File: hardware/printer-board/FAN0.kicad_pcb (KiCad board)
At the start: 2 copper layers, 100 x 100 mm, 12 parts, among them J33 TO FAN0, Q4 D882

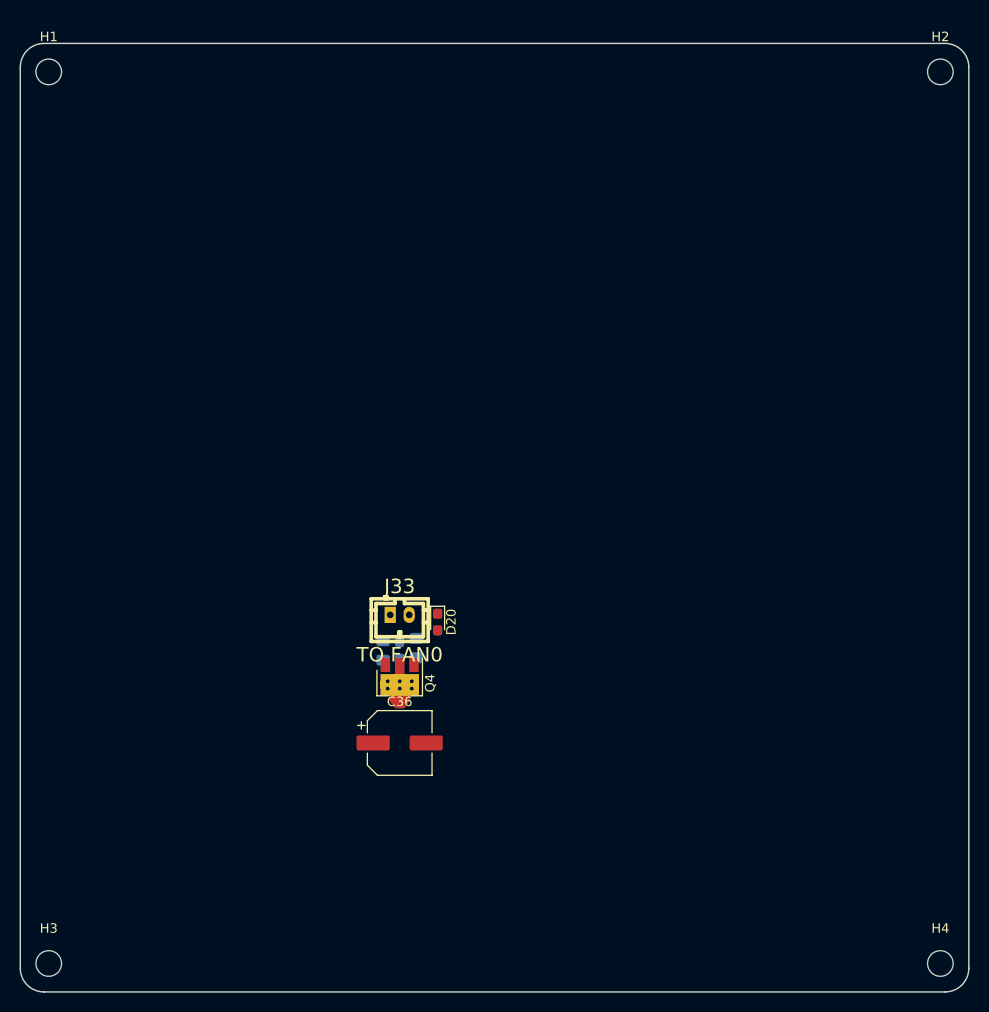
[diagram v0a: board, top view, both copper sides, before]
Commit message: update,
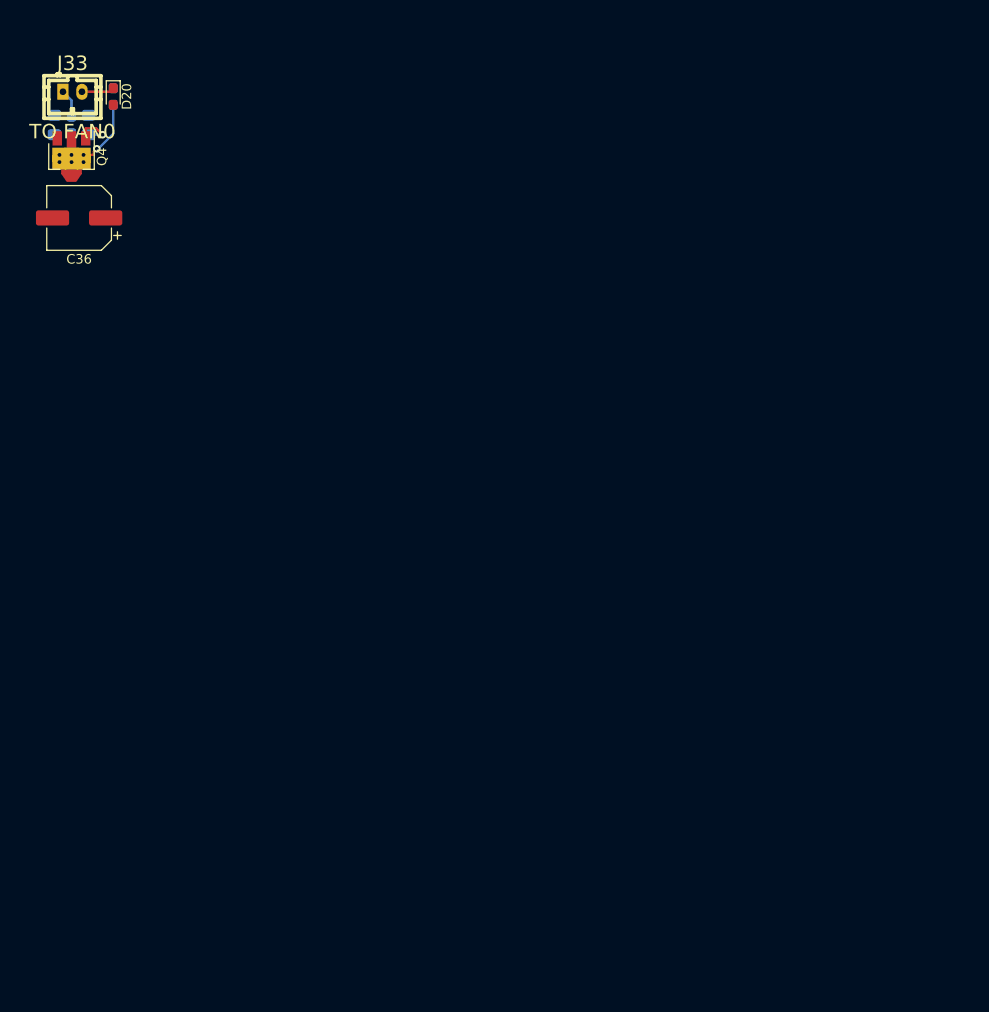
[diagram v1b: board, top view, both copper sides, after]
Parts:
- removed H1, H2, H3, H4: MOUNT_M3, MountingHole:MountingHole_2.7mm_M2.5
- moved R58 65.7 mm to (9.80, 5.60)
- moved Q4 65.4 mm to (5.40, 11.5)
- moved R57 65.3 mm to (3.60, 8.60)
- moved D20 65.1 mm to (9.80, 5.60)
- moved R59 65.1 mm to (5.40, 8.60)
- moved R56 65.1 mm to (7.20, 8.60)
- moved J33 65.1 mm to (5.50, 5.10)
- moved C36 64.9 mm to (6.20, 18.4), turned to 180 degrees
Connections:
- net /FANS/FAN0/FAN_EN renamed /FAN_EN
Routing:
- net Net-(Q4-Pad2): track 0.00 -> 15.4 mm, vias 0 -> 1
- net Net-(D20-Pad1): track 0.00 -> 6.91 mm
- net Net-(Q4-Pad1): track 0.00 -> 4.60 mm, vias 0 -> 1
- net +12V: track 0.00 -> 3.00 mm
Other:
- board outline removed
- rule pad_to_mask_clearance: 0 -> 0.051

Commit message: update,
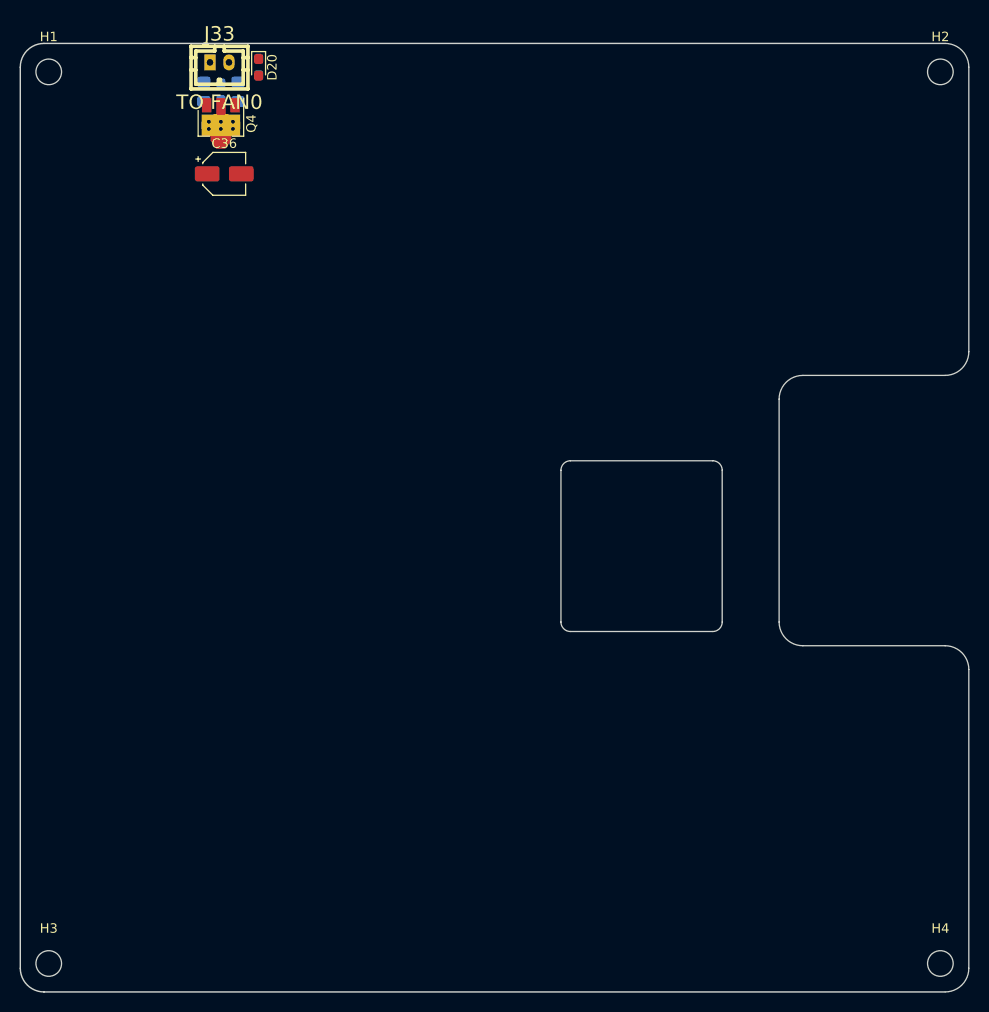
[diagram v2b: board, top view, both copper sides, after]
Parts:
- added H1: MOUNT_M3, MountingHole:MountingHole_2.7mm_M2.5, F.Cu at (3.00, 3.00)
- added H2: MOUNT_M3, MountingHole:MountingHole_2.7mm_M2.5, F.Cu at (97.0, 3.00)
- added H3: MOUNT_M3, MountingHole:MountingHole_2.7mm_M2.5, F.Cu at (3.00, 97.0)
- added H4: MOUNT_M3, MountingHole:MountingHole_2.7mm_M2.5, F.Cu at (97.0, 97.0)
- C36: value CP100uf,16V -> CP1uf,50V; footprint Capacitor_SMD:CP_Elec_6.3x5.3 -> Capacitor_SMD:CP_Elec_4x5.3
- moved R57 16.1 mm to (19.4, 5.10)
- moved Q4 16.1 mm to (21.1, 8.00)
- moved R56 16.1 mm to (22.9, 5.10)
- moved R59 16.1 mm to (21.1, 5.10)
- moved C36 16.0 mm to (21.5, 13.8), turned to 0 degrees
- moved J33 15.8 mm to (21.0, 2.00)
- moved R58 15.6 mm to (25.1, 2.50)
- moved D20 15.6 mm to (25.1, 2.52)
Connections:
- C36 pad 2: GND -> Net-(C36-Pad2)
- D20 pad 1: Net-(D20-Pad1) -> Net-(C36-Pad2)
- J33 pad 2: Net-(D20-Pad1) -> Net-(C36-Pad2)
- R58 pad 1: Net-(D20-Pad1) -> Net-(C36-Pad2)
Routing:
- net Net-(Q4-Pad2): track 15.4 -> 0.00 mm, vias 1 -> 0
- net Net-(D20-Pad1): track 6.91 -> 0.00 mm
- net Net-(Q4-Pad1): track 4.60 -> 0.00 mm, vias 1 -> 0
- net +12V: track 3.00 -> 0.00 mm
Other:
- board outline added: 100 x 100 mm
- rule pad_to_mask_clearance: 0.051 -> 0
